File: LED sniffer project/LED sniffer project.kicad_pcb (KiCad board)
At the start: 2 copper layers, 44 x 52.2 mm, 12 parts, among them J1 Conn_01x02, J2 Conn_01x03, J3 Conn_01x03, J4 Conn_01x04, J5 Conn_01x04, SW1 Push_Button

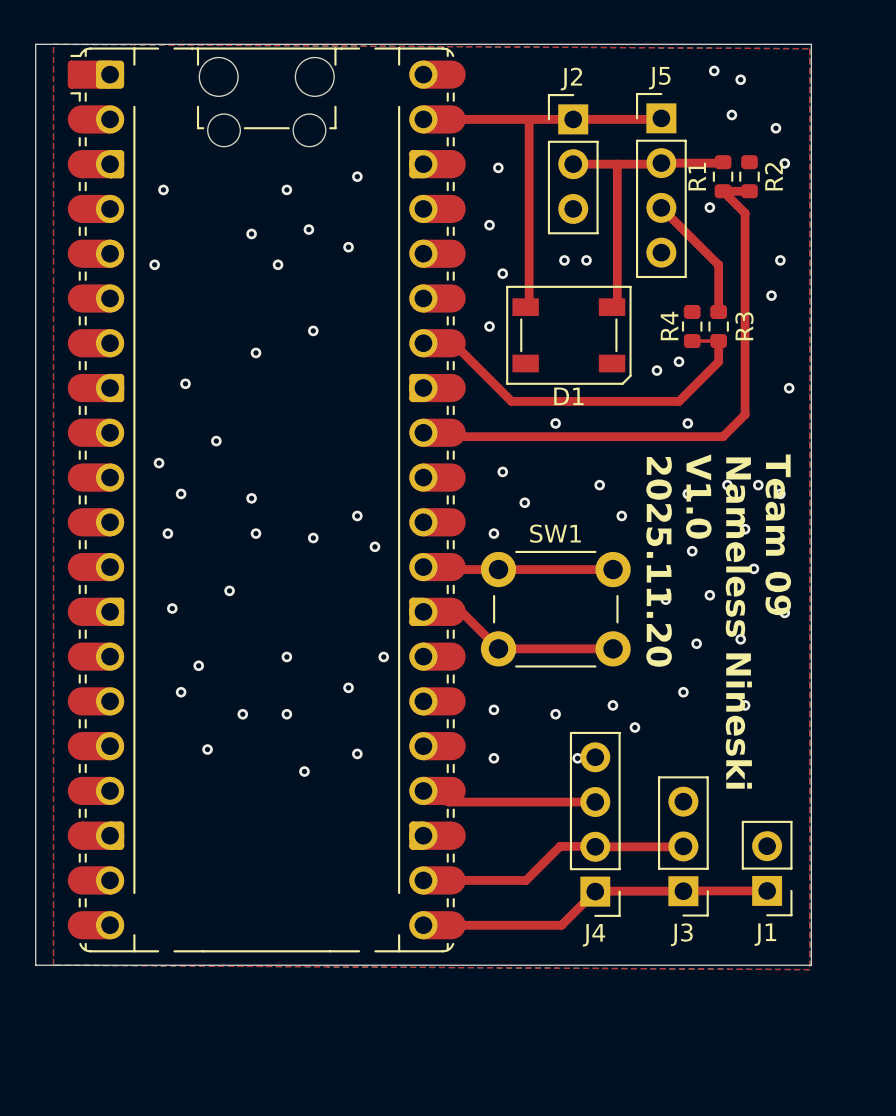
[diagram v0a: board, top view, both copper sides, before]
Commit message: Possible submission
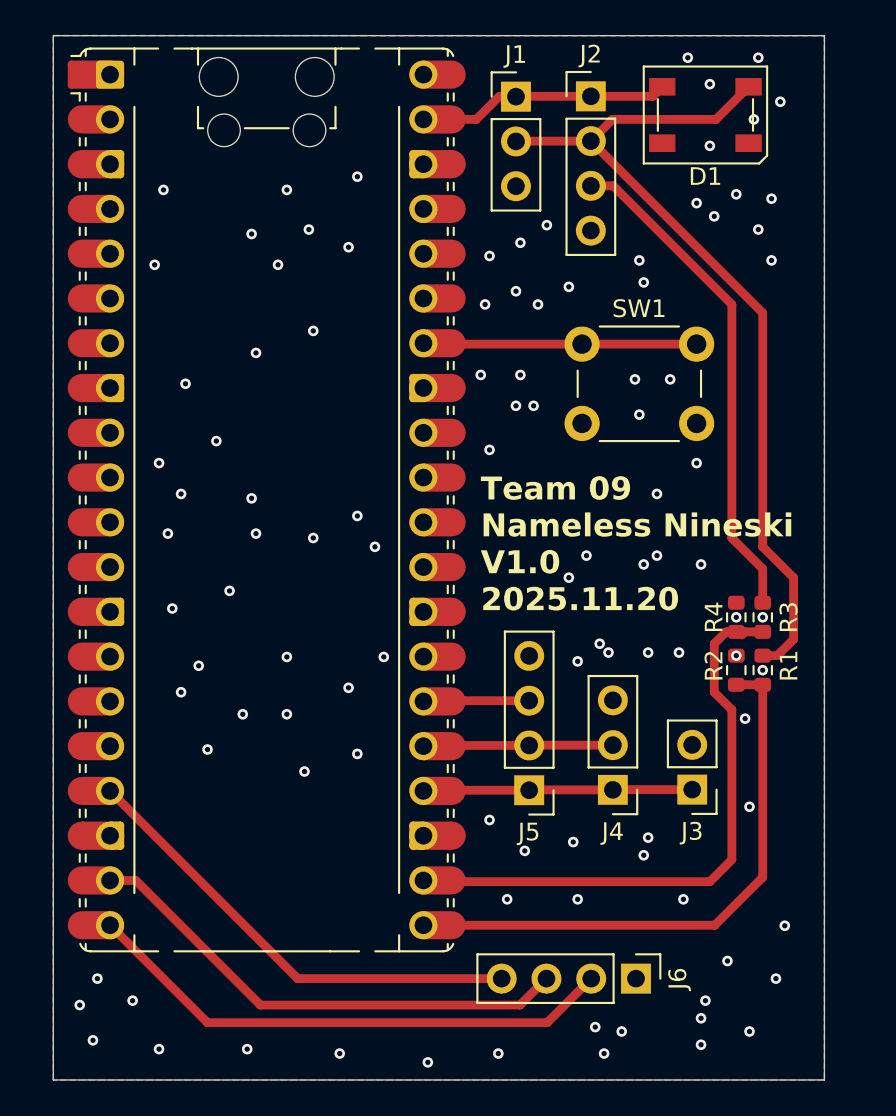
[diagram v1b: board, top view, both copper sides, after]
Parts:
- added J6: Conn_01x04, Connector_PinHeader_2.54mm:PinHeader_1x04_P2.54mm_Vertical, F.Cu at (158.1, 104.2)
- J1: value Conn_01x02 -> Conn_01x03; footprint Connector_PinHeader_2.54mm:PinHeader_1x02_P2.54mm_Vertical -> Connector_PinHeader_2.54mm:PinHeader_1x03_P2.54mm_Vertical
- J2: value Conn_01x03 -> Conn_01x04; footprint Connector_PinHeader_2.54mm:PinHeader_1x03_P2.54mm_Vertical -> Connector_PinHeader_2.54mm:PinHeader_1x04_P2.54mm_Vertical
- J3: value Conn_01x03 -> Conn_01x02; footprint Connector_PinHeader_2.54mm:PinHeader_1x03_P2.54mm_Vertical -> Connector_PinHeader_2.54mm:PinHeader_1x02_P2.54mm_Vertical
- J4: value Conn_01x04 -> Conn_01x03; footprint Connector_PinHeader_2.54mm:PinHeader_1x04_P2.54mm_Vertical -> Connector_PinHeader_2.54mm:PinHeader_1x03_P2.54mm_Vertical
- moved J1 47.3 mm to (151.2, 54.2), turned to 0 degrees
- moved J5 38.9 mm to (152.0, 93.6), turned to 180 degrees
- moved R1 28.1 mm to (165.2, 86.8)
- moved R2 28.0 mm to (163.8, 86.8)
- moved R3 16.7 mm to (165.2, 83.8)
- moved R4 16.7 mm to (163.8, 83.8)
- moved D1 14.7 mm to (162.0, 55.2)
- moved SW1 13.6 mm to (155.0, 68.2)
- moved J4 5.86 mm to (156.8, 93.5)
- moved J3 5.79 mm to (161.2, 93.5)
- moved J2 1.65 mm to (155.5, 54.2)
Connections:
- J1 pad 1: Net-(J1-Pin_1) -> 5V
- J1 pad 2: GND -> Net-(D1-DIN)
- J2 pad 3: GND -> Net-(J2-Pin_3)
- J3 pad 1: Net-(J1-Pin_1) -> Net-(J3-Pin_1)
- J3 pad 2: Net-(J3-Pin_2) -> GND
- J4 pad 1: Net-(J1-Pin_1) -> Net-(J3-Pin_1)
- J4 pad 2: Net-(J3-Pin_2) -> Net-(J4-Pin_2)
- J4 pad 3: Net-(J4-Pin_3) -> GND
- J5 pad 1: 5V -> Net-(J3-Pin_1)
- J5 pad 2: Net-(D1-DIN) -> Net-(J4-Pin_2)
- PICO_MAIN1 pad 17: unconnected-(PICO_MAIN1-GPIO13-Pad17)_1 -> Net-(J6-Pin_4)
- PICO_MAIN1 pad 19: unconnected-(PICO_MAIN1-GPIO14-Pad19) -> Net-(J6-Pin_3)
- PICO_MAIN1 pad 20: unconnected-(PICO_MAIN1-GPIO15-Pad20) -> Net-(J6-Pin_2)
- PICO_MAIN1 pad 21: Net-(J1-Pin_1) -> Net-(PICO_MAIN1-GPIO16)
- PICO_MAIN1 pad 22: Net-(J3-Pin_2) -> Net-(PICO_MAIN1-GPIO17)
- PICO_MAIN1 pad 24: Net-(J4-Pin_3) -> Net-(J3-Pin_1)
- PICO_MAIN1 pad 25: unconnected-(PICO_MAIN1-GPIO19-Pad25) -> Net-(J4-Pin_2)
- PICO_MAIN1 pad 26: unconnected-(PICO_MAIN1-GPIO20-Pad26)_1 -> Net-(J5-Pin_3)
- PICO_MAIN1 pad 29: /BTN_IN -> unconnected-(PICO_MAIN1-GPIO22-Pad29)
- PICO_MAIN1 pad 32: Net-(PICO_MAIN1-GPIO27_ADC1) -> unconnected-(PICO_MAIN1-GPIO27_ADC1-Pad32)_1
- R1 pad 1: Net-(PICO_MAIN1-GPIO27_ADC1) -> Net-(PICO_MAIN1-GPIO16)
- R2 pad 2: Net-(PICO_MAIN1-GPIO27_ADC1) -> Net-(PICO_MAIN1-GPIO16)
- R3 pad 1: Net-(PICO_MAIN1-GPIO28_ADC2) -> Net-(PICO_MAIN1-GPIO17)
- R3 pad 2: Net-(J5-Pin_3) -> Net-(J2-Pin_3)
- R4 pad 2: Net-(PICO_MAIN1-GPIO28_ADC2) -> Net-(PICO_MAIN1-GPIO17)
- SW1 pad 1: /BTN_IN -> Net-(PICO_MAIN1-GPIO28_ADC2)
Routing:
- net Net-(PICO_MAIN1-GPIO17): track 0.00 -> 33.2 mm
- net Net-(D1-DIN): track 16.6 -> 49.7 mm
- net Net-(PICO_MAIN1-GPIO27_ADC1): track 32.8 -> 0.00 mm
- net Net-(PICO_MAIN1-GPIO16): track 0.00 -> 32.0 mm
- net Net-(J6-Pin_2): track 0.00 -> 30.6 mm
- net Net-(J6-Pin_3): track 0.00 -> 29.1 mm
- net Net-(J2-Pin_3): track 0.00 -> 28.4 mm
- net Net-(J6-Pin_4): track 0.00 -> 26.6 mm
- net Net-(J1-Pin_1): track 19.9 -> 0.00 mm
- net Net-(J3-Pin_1): track 0.00 -> 15.3 mm
- net Net-(J3-Pin_2): track 14.8 -> 0.00 mm
- net GND: track 10.8 -> 0.00 mm, vias 76 -> 106
- net Net-(J4-Pin_2): track 0.00 -> 10.8 mm
- net /BTN_IN: track 10.0 -> 0.00 mm
- net Net-(J4-Pin_3): track 9.21 -> 0.00 mm
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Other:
- board size 44 x 52.2 mm -> 43.8 x 59.2 mm
